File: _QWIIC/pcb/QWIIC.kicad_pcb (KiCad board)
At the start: 2 copper layers, 30.5 x 17.8 mm, 19 parts, among them J1 Qwiic, J2 Qwiic, J3 Conn_01x02, J4 Conn_01x02, J5 Conn_01x03, J6 Conn_01x03, U1 ADS1015IDGS, U2 BME280

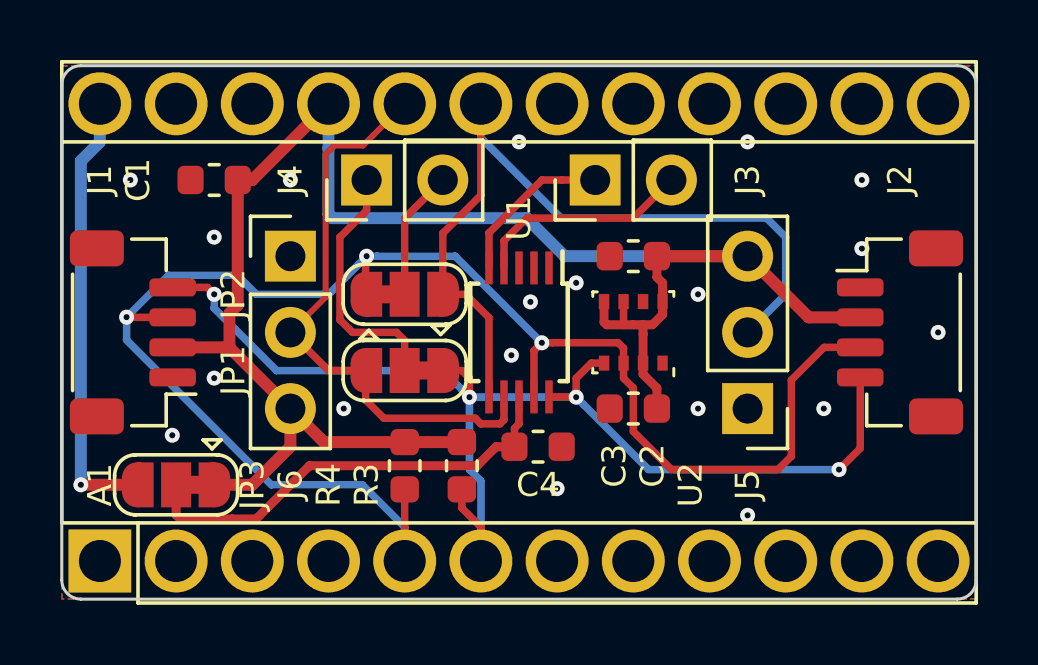
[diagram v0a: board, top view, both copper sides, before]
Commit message: cleanup using licenses
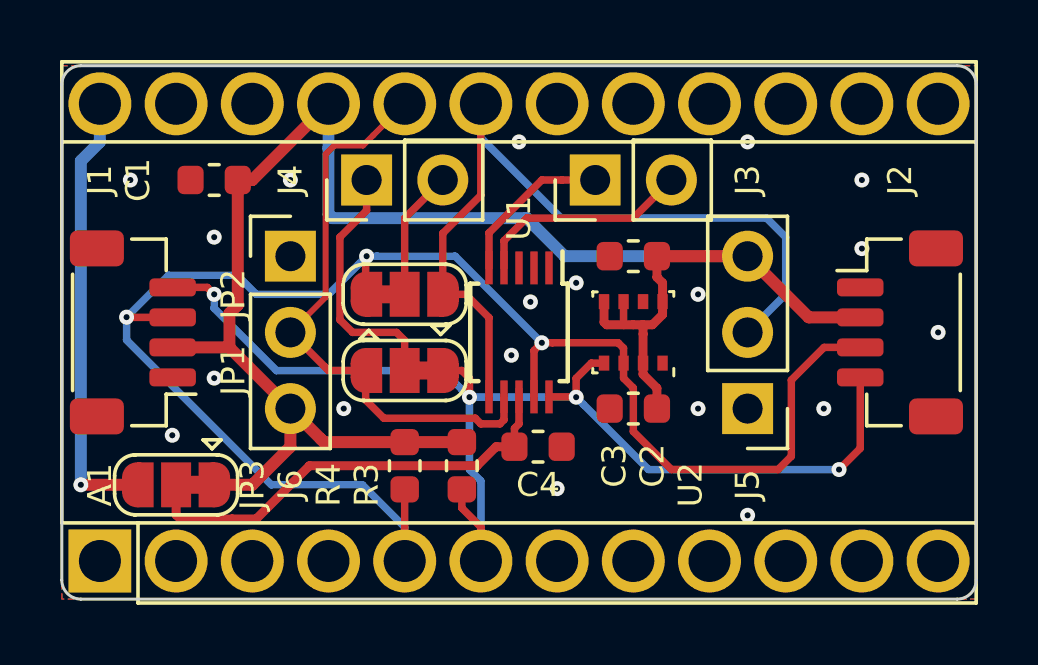
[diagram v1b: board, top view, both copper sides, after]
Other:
- net class Default removed
- net class Power removed
- net class small removed
- net class tiny removed
